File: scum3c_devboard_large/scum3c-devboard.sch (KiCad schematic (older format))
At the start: 34 parts, among them J1 CONSMA001-G, J10 Conn_01x02, J11 Conn_01x01, J3 Conn_02x06_Odd_Even, J5 Conn_02x04_Odd_Even, J6 Conn_01x03, J7 Conn_01x03, J8 Conn_01x03, U1 Perfboard, U12 S-85S1AB18-I6T1U, U5 ICM-20948, U6 S-85S1AB10-I6T1U, U7 S-85S1AB15-I6T1U

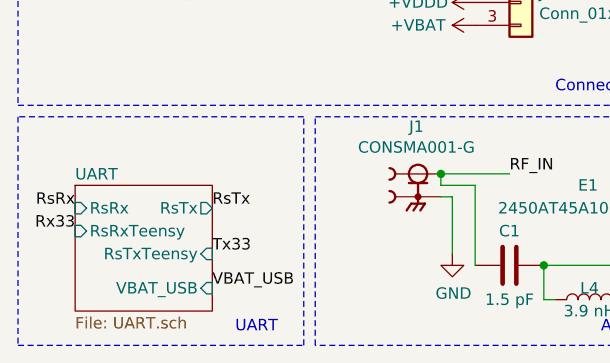
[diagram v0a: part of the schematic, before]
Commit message: ensuring large board up to date with master
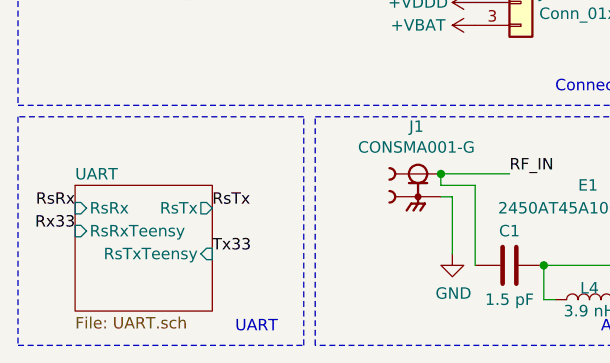
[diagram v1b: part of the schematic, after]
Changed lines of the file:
@@
 F2 "RsRx" I L 800 7200 50
 F3 "RsTx" O R 1400 7200 50
-F4 "VBAT_USB" I R 1400 7550 50
 F5 "RsTxTeensy" I R 1400 7400 50
 F6 "RsRxTeensy" I L 800 7300 50
@@
 	1    0    0    -1
 $EndComp
-Text Label 1400 7550 0    50   ~ 0
-VBAT_USB
 $Comp
 L Connector_Generic:Conn_01x03 J8
